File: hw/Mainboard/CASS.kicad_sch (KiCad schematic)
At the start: 16 parts, among them J5 CASS A, J6 CASS B, Q1 AO3401A, Q3 AO3401A

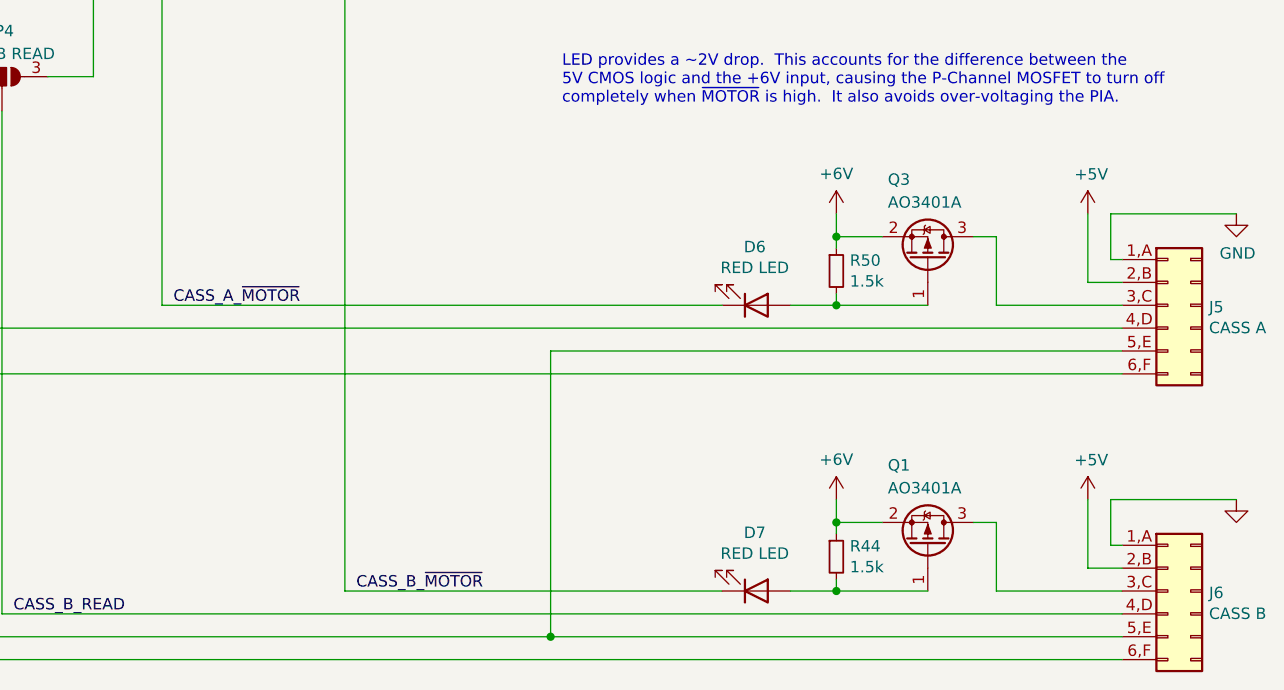
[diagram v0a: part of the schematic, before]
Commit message: hw: wip add MCU, 2 layer board
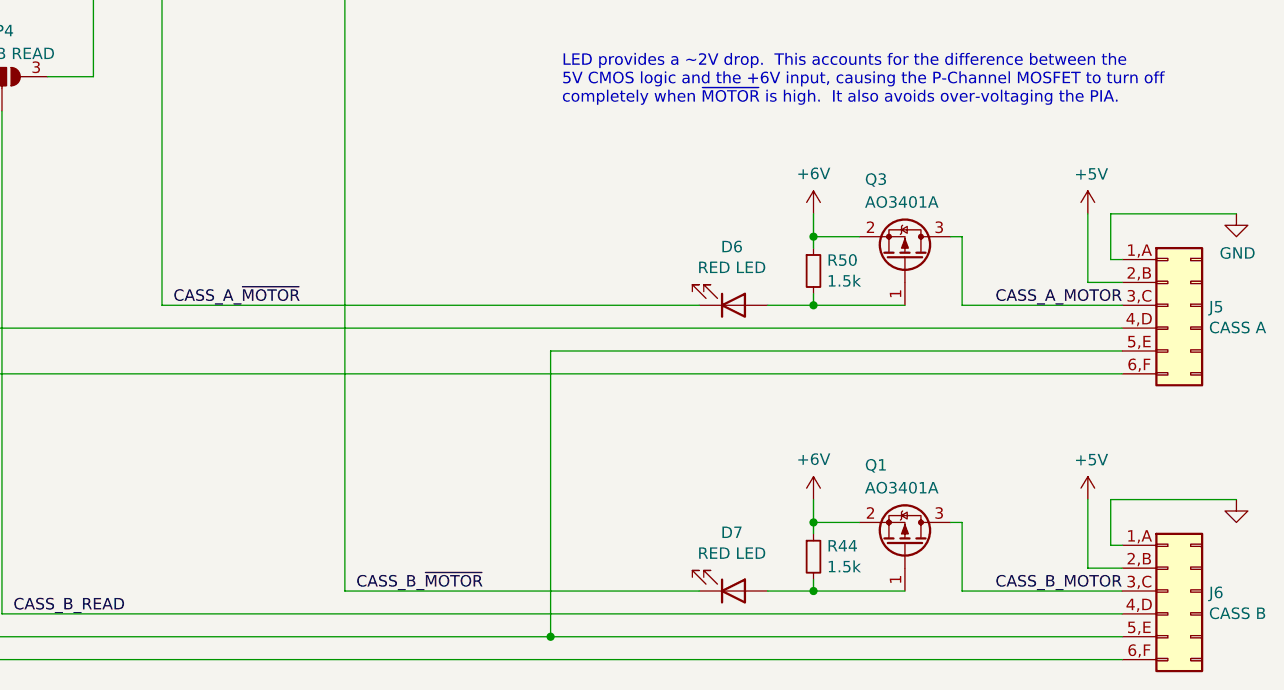
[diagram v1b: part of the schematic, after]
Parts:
- J5, J6: footprint PET:EDGE_CON_12P_TAPE -> Retrocomputing:CBM_PET_CASS_EDGE_CON_12P; symbol Mainboard-rescue:Conn_01x06_Card_Edge-PET -> Retrocomputing:CBM_PET_CASS_Conn_01x06_Card_Edge
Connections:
- net CASS_B_MOTOR: now reaches J6.3,C (MOTOR), Q1.3 (D)
- net CASS_A_MOTOR: now reaches J5.3,C (MOTOR), Q3.3 (D)
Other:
- moved on the sheet: D6, D7, Q1, Q3, R44, R50
